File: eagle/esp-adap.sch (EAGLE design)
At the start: 3 parts

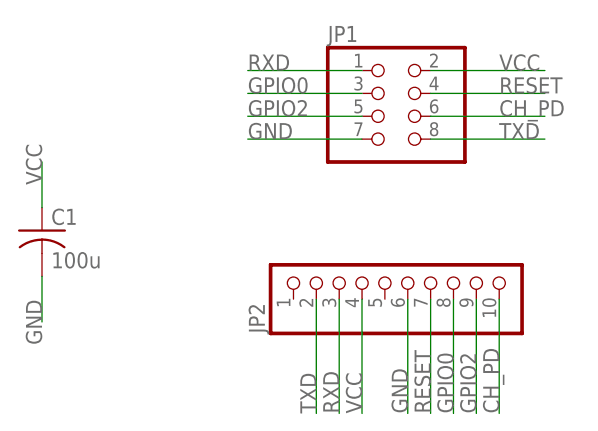
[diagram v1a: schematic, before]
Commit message: changed header
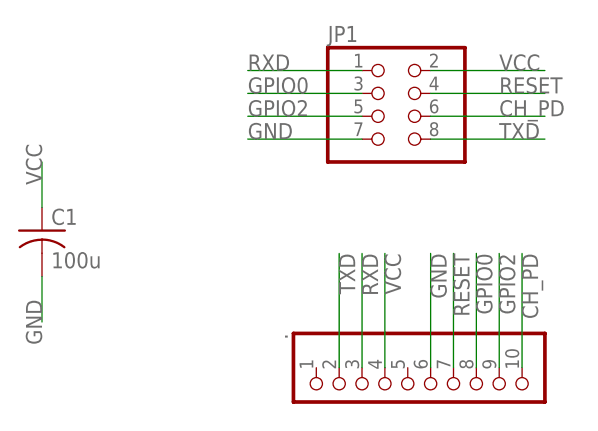
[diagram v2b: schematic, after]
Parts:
- removed JP2: (no value), pinhead:PINHD-1X10
- added .: (no value), pinhead:PINHD-1X10
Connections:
- net CH_PD: now also ..10; no longer JP2.10
- net GND: now also ..6; no longer JP2.6
- net GPIO0: now also ..8; no longer JP2.8
- net GPIO2: now also ..9; no longer JP2.9
- net RESET: now also ..7; no longer JP2.7
- net RXD: now also ..3; no longer JP2.3
- net TXD: now also ..2; no longer JP2.2
- net VCC: now also ..4; no longer JP2.4
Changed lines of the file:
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@@
 <parts>
 <part name="JP1" library="pinhead" deviceset="PINHD-2X4" device=""/>
-<part name="JP2" library="pinhead" deviceset="PINHD-1X10" device=""/>
+<part name="." library="pinhead" deviceset="PINHD-1X10" device=""/>
 <part name="C1" library="resistor" deviceset="C-US" device="C1206K" value="100u"/>
 </parts>
@@
 <instances>
 <instance part="JP1" gate="A" x="40.64" y="40.64"/>
-<instance part="JP2" gate="A" x="40.64" y="22.86" rot="R90"/>
+<instance part="." gate="A" x="43.18" y="10.16" rot="MR270"/>
 <instance part="C1" gate="G$1" x="2.54" y="27.94"/>
 </instances>
@@
 </segment>
 <segment>
-<pinref part="JP2" gate="A" pin="3"/>
-<wire x1="35.56" y1="20.32" x2="35.56" y2="7.62" width="0.1524" layer="91"/>
-<label x="35.56" y="7.62" size="1.778" layer="95" rot="R90"/>
+<pinref part="." gate="A" pin="3"/>
+<wire x1="38.1" y1="12.7" x2="38.1" y2="25.4" width="0.1524" layer="91"/>
+<label x="38.1" y="25.4" size="1.778" layer="95" rot="R270"/>
 </segment>
 </net>
@@
 </segment>
 <segment>
-<pinref part="JP2" gate="A" pin="8"/>
-<wire x1="48.26" y1="20.32" x2="48.26" y2="7.62" width="0.1524" layer="91"/>
-<label x="48.26" y="7.62" size="1.778" layer="95" rot="R90"/>
+<pinref part="." gate="A" pin="8"/>
+<wire x1="50.8" y1="12.7" x2="50.8" y2="25.4" width="0.1524" layer="91"/>
+<label x="50.8" y="25.4" size="1.778" layer="95" rot="R270"/>
 </segment>
 </net>
@@
 </segment>
 <segment>
-<pinref part="JP2" gate="A" pin="9"/>
-<wire x1="50.8" y1="20.32" x2="50.8" y2="7.62" width="0.1524" layer="91"/>
-<label x="50.8" y="7.62" size="1.778" layer="95" rot="R90"/>
+<pinref part="." gate="A" pin="9"/>
+<wire x1="53.34" y1="12.7" x2="53.34" y2="25.4" width="0.1524" layer="91"/>
+<label x="53.34" y="25.4" size="1.778" layer="95" rot="R270"/>
 </segment>
 </net>
@@
 </segment>
 <segment>
-<pinref part="JP2" gate="A" pin="7"/>
-<wire x1="45.72" y1="20.32" x2="45.72" y2="7.62" width="0.1524" layer="91"/>
-<label x="45.72" y="7.62" size="1.778" layer="95" rot="R90"/>
+<pinref part="." gate="A" pin="7"/>
+<wire x1="48.26" y1="12.7" x2="48.26" y2="25.4" width="0.1524" layer="91"/>
+<label x="48.26" y="25.4" size="1.778" layer="95" rot="R270"/>
 </segment>
 </net>
@@
 </segment>
 <segment>
-<pinref part="JP2" gate="A" pin="10"/>
-<wire x1="53.34" y1="20.32" x2="53.34" y2="7.62" width="0.1524" layer="91"/>
-<label x="53.34" y="7.62" size="1.778" layer="95" rot="R90"/>
+<pinref part="." gate="A" pin="10"/>
+<wire x1="55.88" y1="12.7" x2="55.88" y2="25.4" width="0.1524" layer="91"/>
+<label x="55.88" y="25.4" size="1.778" layer="95" rot="R270"/>
 </segment>
 </net>
@@
 </segment>
 <segment>
-<pinref part="JP2" gate="A" pin="2"/>
-<wire x1="33.02" y1="20.32" x2="33.02" y2="7.62" width="0.1524" layer="91"/>
-<label x="33.02" y="7.62" size="1.778" layer="95" rot="R90"/>
+<pinref part="." gate="A" pin="2"/>
+<wire x1="35.56" y1="12.7" x2="35.56" y2="25.4" width="0.1524" layer="91"/>
+<label x="35.56" y="25.4" size="1.778" layer="95" rot="R270"/>
 </segment>
 </net>
@@
 </segment>
 <segment>
-<pinref part="JP2" gate="A" pin="4"/>
-<wire x1="38.1" y1="20.32" x2="38.1" y2="7.62" width="0.1524" layer="91"/>
-<label x="38.1" y="7.62" size="1.778" layer="95" rot="R90"/>
+<pinref part="." gate="A" pin="4"/>
+<wire x1="40.64" y1="12.7" x2="40.64" y2="25.4" width="0.1524" layer="91"/>
+<label x="40.64" y="25.4" size="1.778" layer="95" rot="R270"/>
 </segment>
 </net>
@@
 </segment>
 <segment>
-<pinref part="JP2" gate="A" pin="6"/>
-<wire x1="43.18" y1="20.32" x2="43.18" y2="7.62" width="0.1524" layer="91"/>
-<label x="43.18" y="7.62" size="1.778" layer="95" rot="R90"/>
+<pinref part="." gate="A" pin="6"/>
+<wire x1="45.72" y1="12.7" x2="45.72" y2="25.4" width="0.1524" layer="91"/>
+<label x="45.72" y="25.4" size="1.778" layer="95" rot="R270"/>
 </segment>
 </net>
